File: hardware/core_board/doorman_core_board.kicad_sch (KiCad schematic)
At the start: 57 parts, among them J1 USB-C Connector, J10 VCC Test Pad, J2 Screw Terminals, J3 3V3 Test Pad, J4 Extension Board Connector, J5 Siedle BUS RX Test Pad, J6 BUS Test Pad, J7 BUS RX Test Pad, J8 TX Test Pad, J9 RX Test Pad, Q1 BC847BPN, Q2 BC817-40, Q3 BC817-40, Q4 BC817-40, Q6 BC847BPN, SW1 Button, SW2 Button, U2 AP63203WU, U3 GAQY252G3S, U4 ESP32-S3-MINI-1

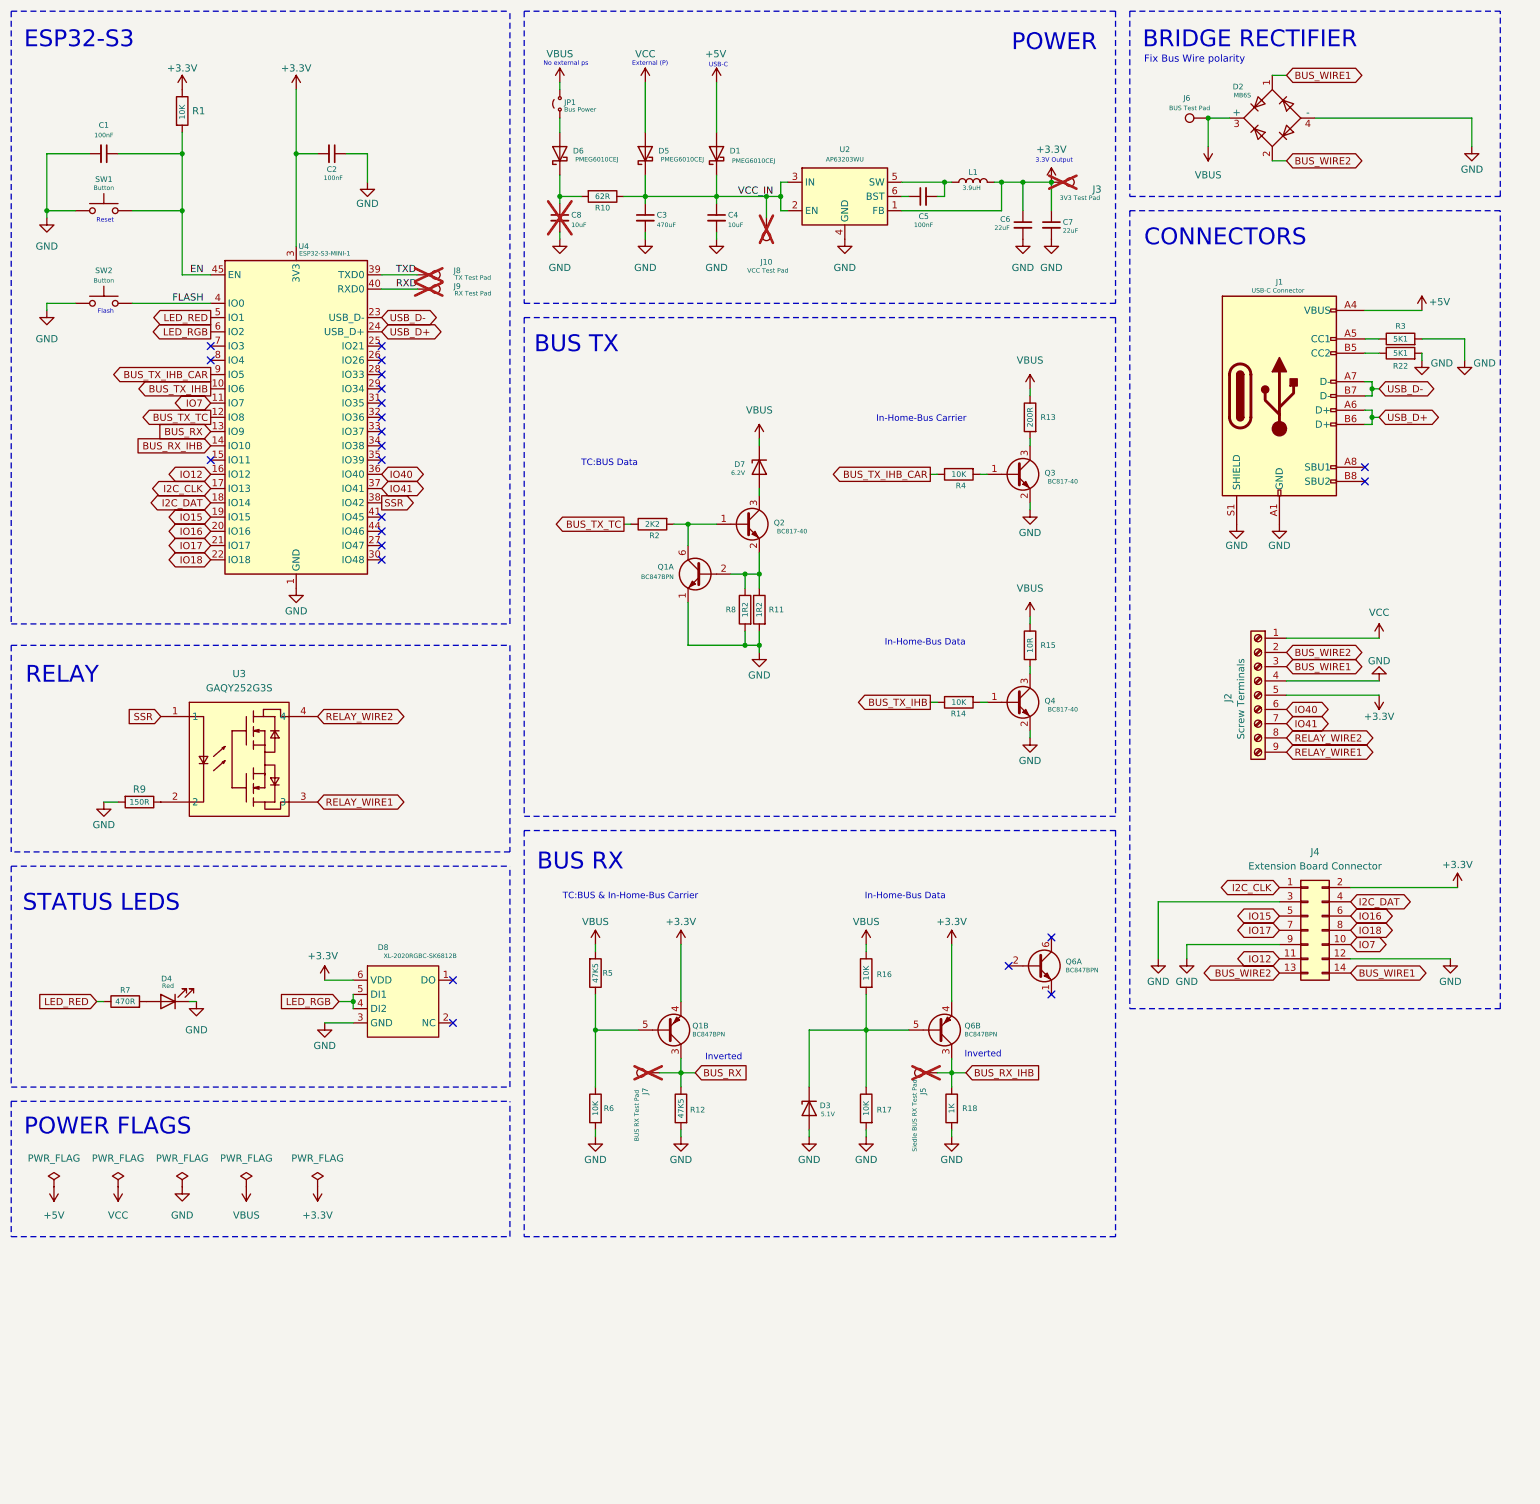
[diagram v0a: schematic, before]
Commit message: Change structure
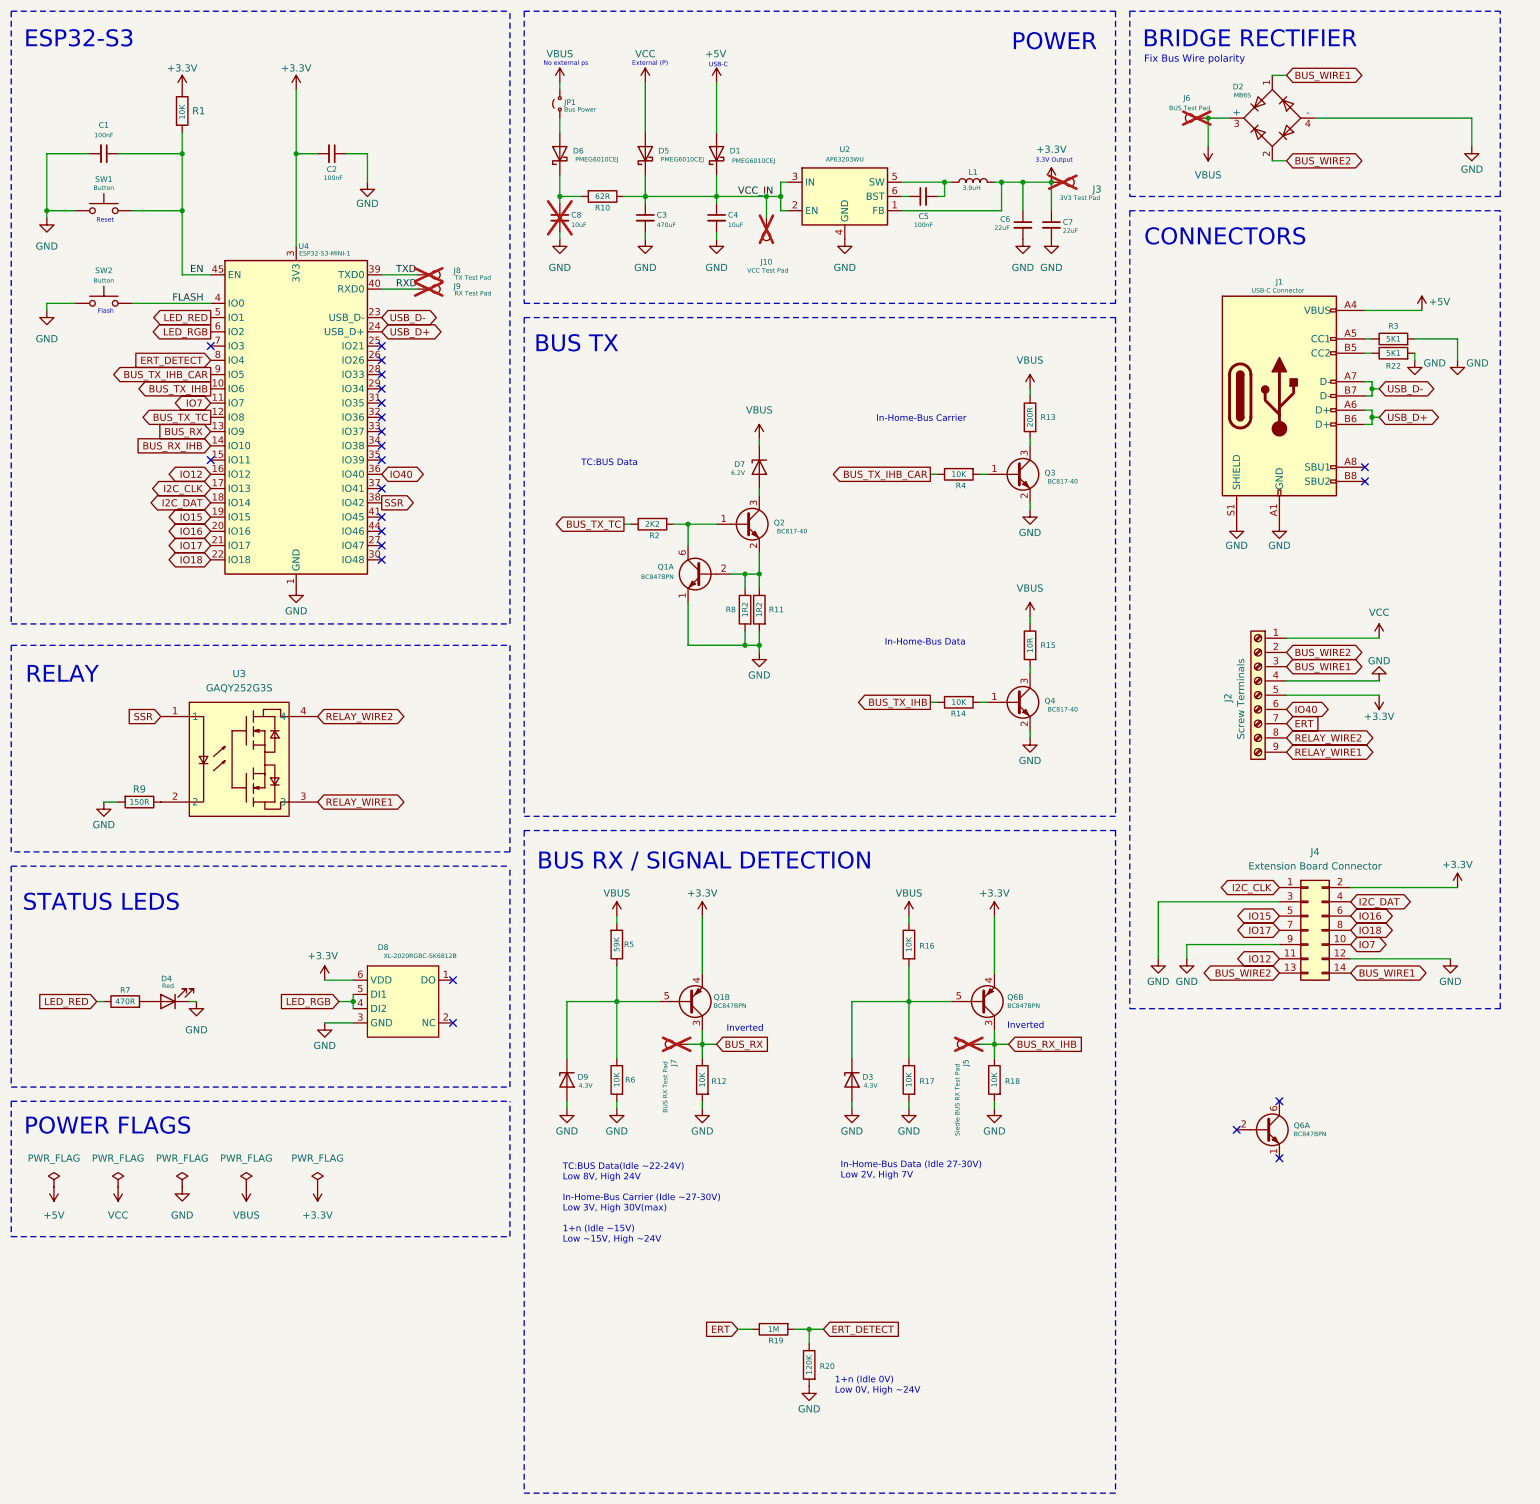
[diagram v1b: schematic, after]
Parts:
- added D9: 4.3V, Diode_SMD:D_SOD-123, symbol Diode:BZV55C6V2
- added R19: 1M, Resistor_SMD:R_0603_1608Metric, symbol Device:R
- added R20: 120K, Resistor_SMD:R_0603_1608Metric, symbol Device:R
- D3: value 5.1V -> 4.3V; LCSC C85181 -> C19077399; MPN MMSZ5231B-7-F -> BZT52C4V3
- J6: now not fitted
- R11, R8: LCSC C5140149 -> C17381; MPN SCR0805J1R2 -> 0805W8F120KT5E
- R12: value 47K5 -> 10K; LCSC C23061 -> C25804; MPN 0603WAF4752T5E -> 0603WAF1002T5E
- R18: value 1K -> 10K; footprint Resistor_SMD:R_0402_1005Metric -> Resistor_SMD:R_0603_1608Metric; LCSC C11702 -> C25804; MPN 0402WGF1001TCE -> 0603WAF1002T5E; Package 0402 -> 0603
- R5: value 47K5 -> 59K; LCSC C23061 -> C23085; MPN 0603WAF4752T5E -> 0603WAF5902T5E
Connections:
- net GND: now also D9.2 (A), R20.2
- net at Q1.5 (B2), R5.1, R6.1: now also D9.1 (K)
- net ERT_DETECT: now reaches U4.8 (IO4)
- net ERT_DETECT: now also R19.2, R20.1
- net IO41: no longer names the net of U4.37 (IO41)
- net IO41: no longer J2.7 (Pin_7)
- new net ERT: J2.7 (Pin_7), R19.1
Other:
- note added: "1+n (Idle 0V) Low 0V, High ~24V"
- note added: "BUS RX / SIGNAL DETECTION"
- note added: "In-Home-Bus Data (Idle 27-30V) Low 2V, High 7V"
- note added: "TC:BUS Data(Idle ~22-24V) Low 8V, High 24V In-Home-Bus Carrier (Idle ~27-30V) Low 3V, High 30V(max) 1+n (Idle ~15V) Low ~15V, High ~24V"
- note removed: "BUS RX"
- note removed: "TC:BUS & In-Home-Bus Carrier"
- moved on the sheet: D3, J5, J7, Q1B, Q6A, Q6B, R12, R16, R17, R22, R3, R5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

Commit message: WIP
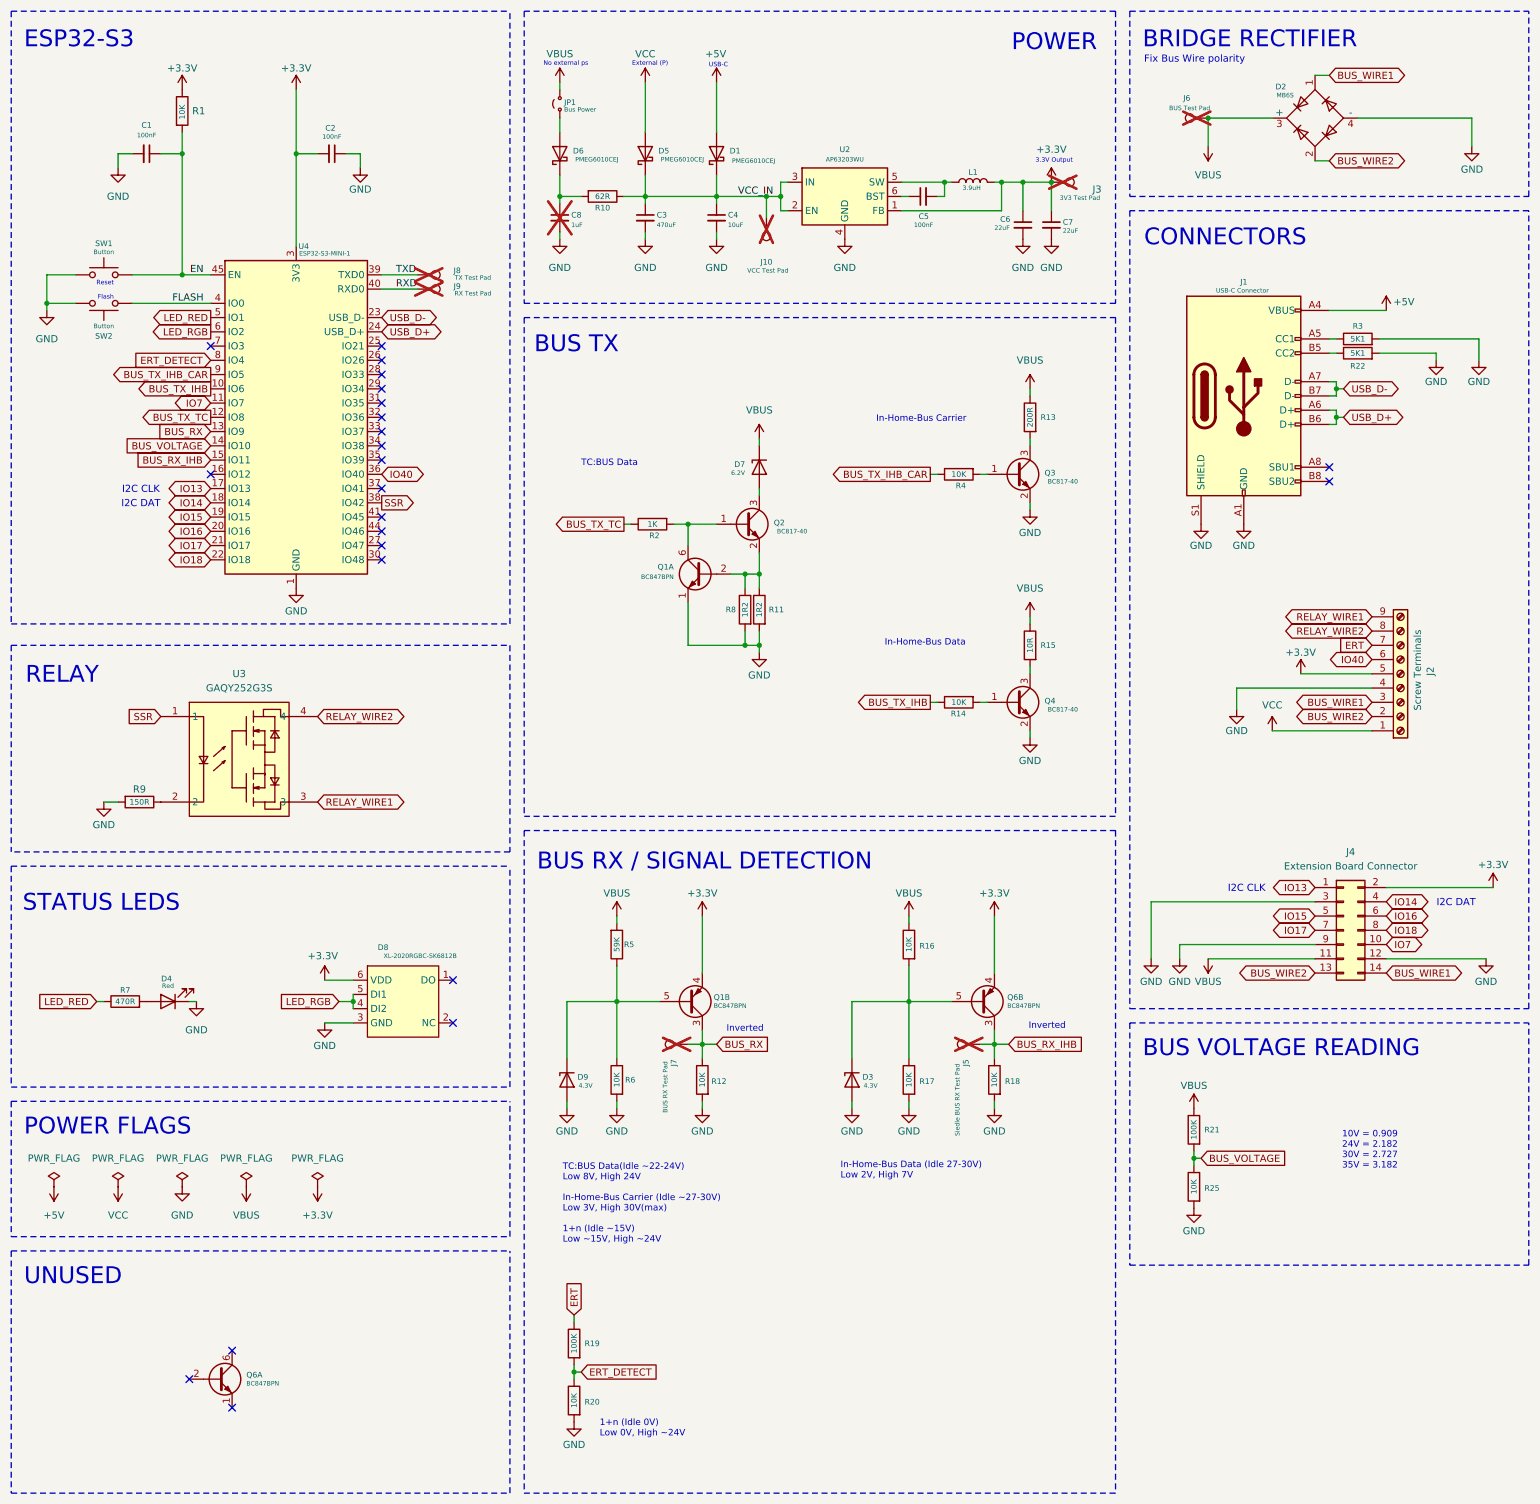
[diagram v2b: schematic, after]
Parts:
- added R21: 100K, Resistor_SMD:R_0603_1608Metric, symbol Device:R
- added R25: 10K, Resistor_SMD:R_0603_1608Metric, symbol Device:R
- C8: value 10uF -> 1uF; LCSC C89632 -> C1848; MPN CL31B106KBHNNNE -> CL31B105KBHNNNE
- R13: LCSC C25361 -> C2765758; MPN 1206W4J0201T5E -> HP06W2F2000T5E
- R15: LCSC C17903 -> C511457; MPN 1206W4F100JT5E -> CRCW120610R0FKEAHP
- R19: value 1M -> 100K; LCSC C22935 -> C25803; MPN 0603WAF1004T5E -> 0603WAF1003T5E
- R2: value 2K2 -> 1K; LCSC C25879 -> C11702; MPN 0402WGF2201TCE -> 0402WGF1001TCE
- R20: value 120K -> 10K; LCSC C25808 -> C25804; MPN 0603WAF1203T5E -> 0603WAF1002T5E
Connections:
- net BUS_RX_IHB: now also U4.15 (IO11); no longer U4.14 (IO10)
- net GND: now also R25.2
- net VBUS: now also J4.11 (Pin_11), R21.1
- net I2C_CLK renamed IO13
- net I2C_DAT renamed IO14
- net IO12: no longer names the net of U4.16 (IO12)
- net IO12: no longer J4.11 (Pin_11)
- new net BUS_VOLTAGE: R21.2, R25.1, U4.14 (IO10)
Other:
- note added: "10V = 0.909 24V = 2.182 30V = 2.727 35V = 3.182"
- note added: "BUS VOLTAGE READING"
- note added: "I2C CLK"
- note added: "I2C DAT"
- note added: "UNUSED"
- moved on the sheet: C1, D2, J1, J2, J4, Q6A, R19, R20, R22, R3, SW1, SW2
